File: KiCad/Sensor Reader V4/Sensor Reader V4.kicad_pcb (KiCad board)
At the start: 2 copper layers, 51.5 x 63 mm, 71 parts, among them IC1 TLV76733DGNR, IC2 ESP32-C3-WROOM-02-H4, J1 USB_C_Receptacle_USB2.0_16P, J10 L_I/B1_Out, J11 B1_Net/B2_In, J12 B2_Net/B2_Out, J13 AIN_4, J14 AIN_5, J15 5V_Input, J16 3.3V_Output, J2 GPIO, J6 Exposed_UART, J7 Batt1_V, J8 Batt2_V, J9 M_OUT/B1_In, SW1 BOOT_Btn, SW2 EN_Btn, U3 ADS8688

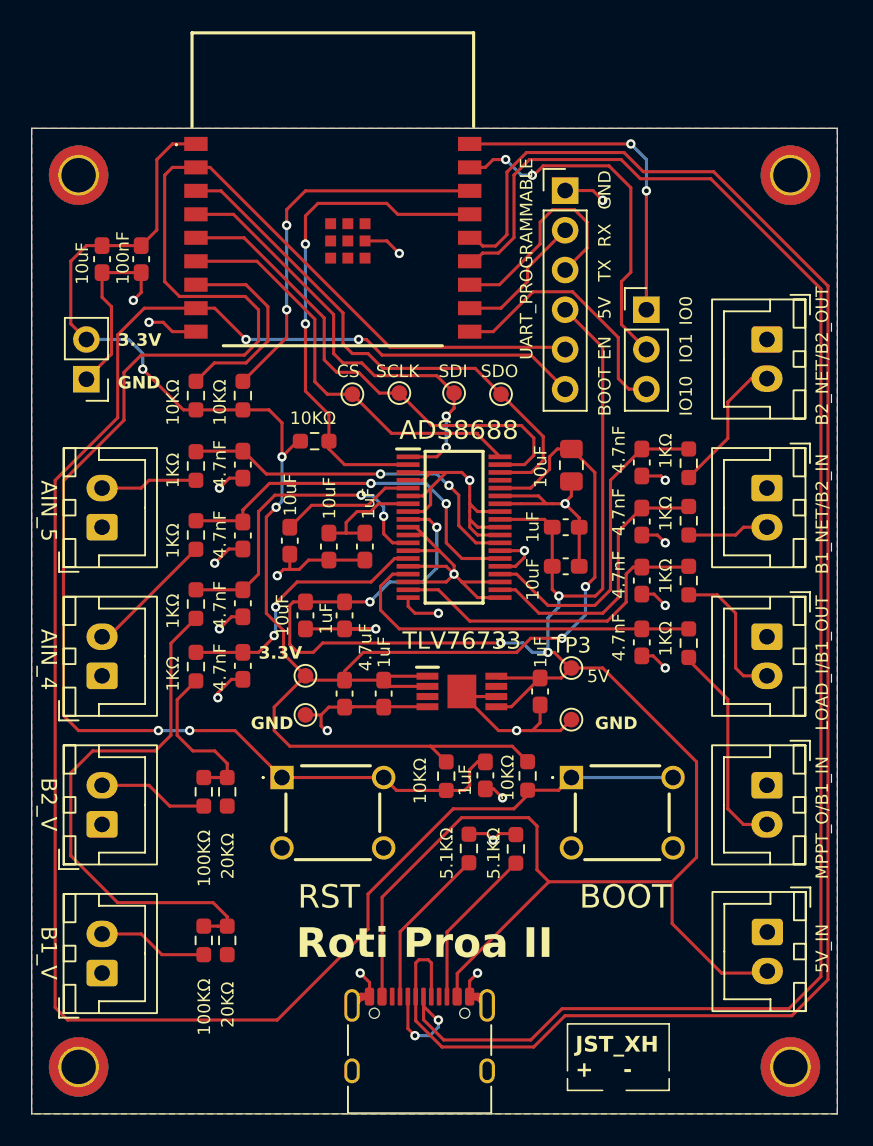
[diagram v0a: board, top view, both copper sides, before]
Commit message: update
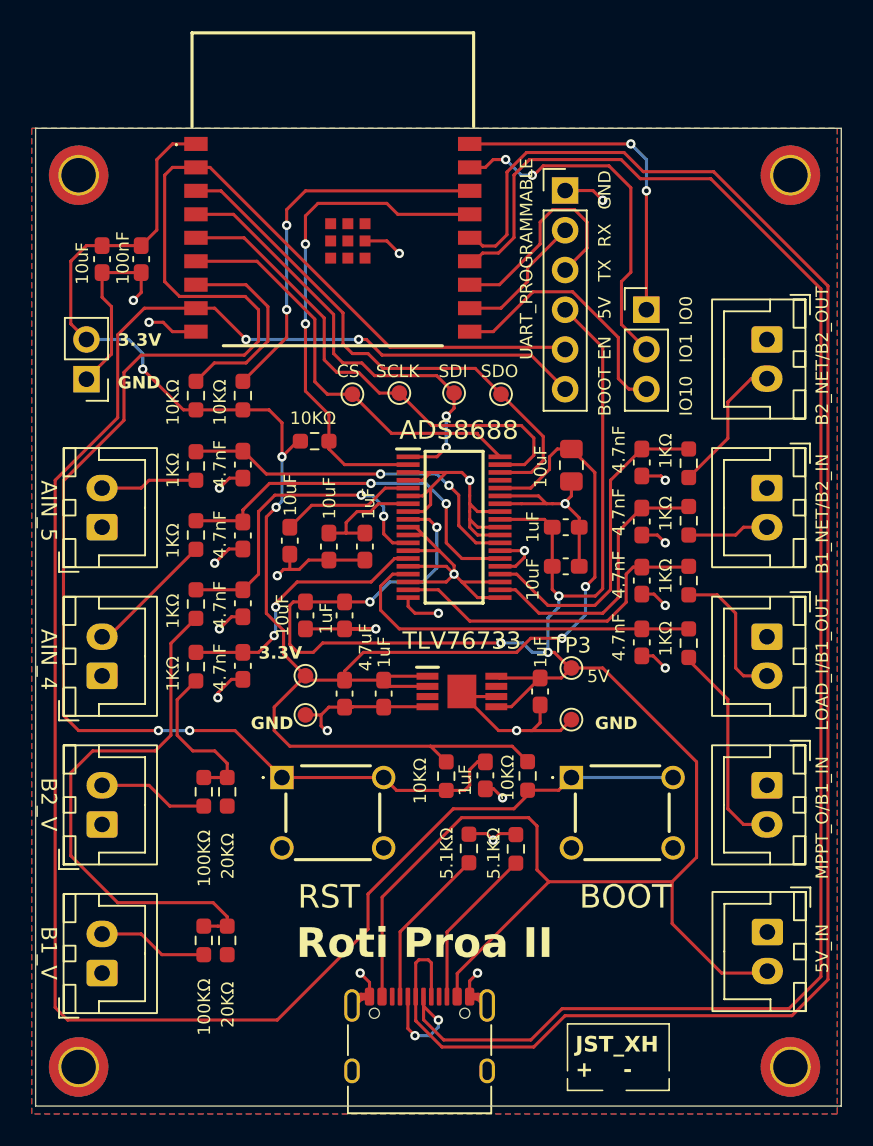
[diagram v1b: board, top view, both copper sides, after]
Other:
- board size 51.5 x 63 mm -> 51.5 x 62.5 mm
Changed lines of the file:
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@@
 	)
 	(gr_rect
-		(start 117.5 38)
-		(end 169 101)
+		(start 117.75 38)
+		(end 169.25 100.5)
 		(stroke
 			(width 0.05)
